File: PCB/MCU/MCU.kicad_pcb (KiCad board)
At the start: 2 copper layers, 40 x 46.2 mm, 36 parts, among them IC1 TMP112NAIDRLR, J1 Conn_02x06_Odd_Even, J2 Conn_02x06_Odd_Even, J3 USB_B_Micro, J4 Programmer, SW1 SW_Push, U1 MPU6050, U2 MDBT50Q-1MV2, U3 MAX6372, Y1 32.768kHz

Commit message: udated by FZ from Windows
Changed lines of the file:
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@@
     (grid_origin 150.16 123.198621)
     (pcbplotparams
-      (layerselection 0x0000020_7ffffffe)
+      (layerselection 0x00010fc_ffffffff)
       (plot_on_all_layers_selection 0x0000000_00000000)
       (disableapertmacros false)
@@
       (sketchpadsonfab false)
       (subtractmaskfromsilk false)
-      (outputformat 3)
+      (outputformat 1)
       (mirror false)
       (drillshape 0)
       (scaleselection 1)
-      (outputdirectory "./")
+      (outputdirectory "Gerber/")
     )
   )
@@
     (fp_line (start 1 0.625) (end -1 0.625)
       (stroke (width 0.1) (type solid)) (layer "F.Fab"))
-    (pad "1" smd roundrect (at -1.0375 0 270) (size 1.175 1.45) (layers "F.Cu" "F.Paste" "F.Mask") (roundrect_rratio 0.212766)
+    (pad "1" smd roundrect (at -1.0375 0 270) (size 1.175 1.45) (layers "F.Cu" "F.Paste" "F.Mask") (roundrect_rratio 0.2127659574)
       (net 7 "+5V") (pintype "passive"))
-    (pad "2" smd roundrect (at 1.0375 0 270) (size 1.175 1.45) (layers "F.Cu" "F.Paste" "F.Mask") (roundrect_rratio 0.212766)
+    (pad "2" smd roundrect (at 1.0375 0 270) (size 1.175 1.45) (layers "F.Cu" "F.Paste" "F.Mask") (roundrect_rratio 0.2127659574)
       (net 1 "GND") (pintype "passive"))
     (model "${KICAD6_3DMODEL_DIR}/Capacitor_SMD.3dshapes/C_0805_2012Metric.wrl"
@@
     (fp_line (start 1 0.625) (end -1 0.625)
       (stroke (width 0.1) (type solid)) (layer "F.Fab"))
-    (pad "1" smd roundrect (at -1.0375 0 270) (size 1.175 1.45) (layers "F.Cu" "F.Paste" "F.Mask") (roundrect_rratio 0.212766)
+    (pad "1" smd roundrect (at -1.0375 0 270) (size 1.175 1.45) (layers "F.Cu" "F.Paste" "F.Mask") (roundrect_rratio 0.2127659574)
       (net 4 "Net-(U2-P0.01{slash}XL2)") (pinfunction "1") (pintype "passive"))
-    (pad "2" smd roundrect (at 1.0375 0 270) (size 1.175 1.45) (layers "F.Cu" "F.Paste" "F.Mask") (roundrect_rratio 0.212766)
+    (pad "2" smd roundrect (at 1.0375 0 270) (size 1.175 1.45) (layers "F.Cu" "F.Paste" "F.Mask") (roundrect_rratio 0.2127659574)
       (net 3 "Net-(U2-P0.00{slash}XL1)") (pinfunction "2") (pintype "passive"))
     (model "${KICAD6_3DMODEL_DIR}/Capacitor_SMD.3dshapes/C_0805_2012Metric.wrl"

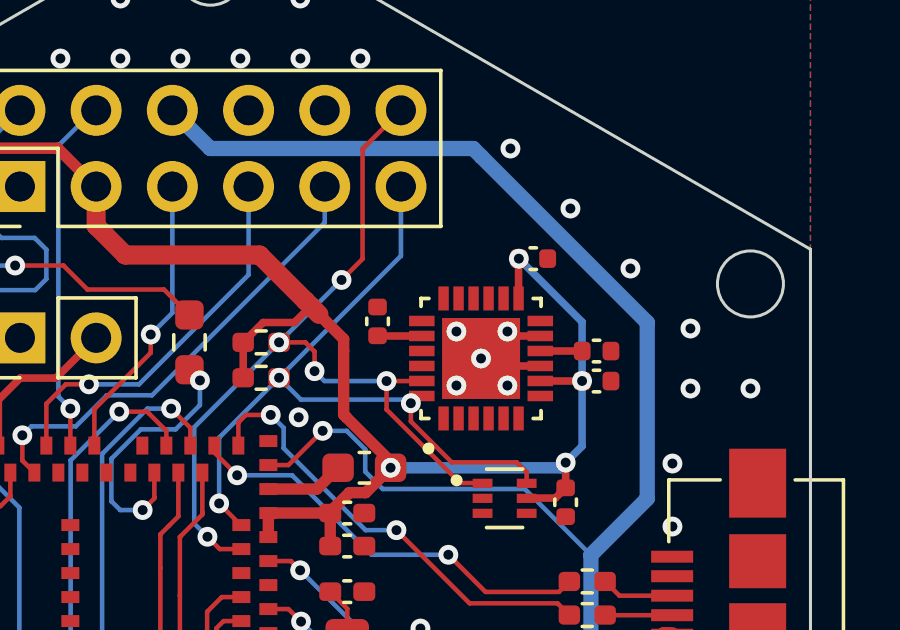
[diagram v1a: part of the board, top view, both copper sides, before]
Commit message: udated by FZ from Windows
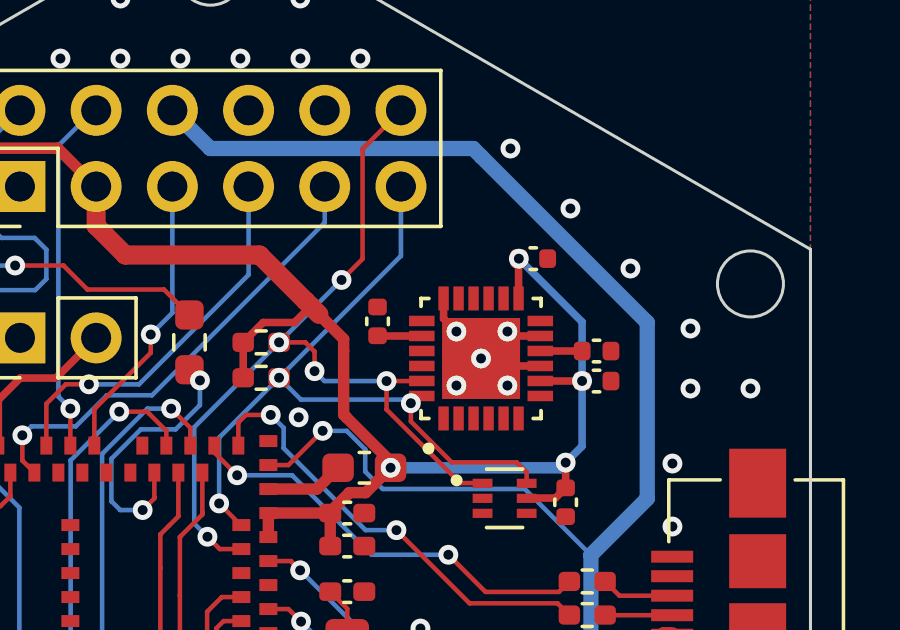
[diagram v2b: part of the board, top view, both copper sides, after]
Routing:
- net GND: track 3.24 -> 4.51 mm
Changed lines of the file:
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@@
   (segment (start 161.155 92.4475) (end 159.43 92.4475) (width 0.254) (layer "F.Cu") (net 1))
   (segment (start 160.208879 91.4475) (end 160.06 91.298621) (width 0.254) (layer "F.Cu") (net 1))
+  (segment (start 157.93 90.1975) (end 157.93 90.868621) (width 0.254) (layer "F.Cu") (net 1))
   (segment (start 159.43 92.4475) (end 159.18 92.1975) (width 0.254) (layer "F.Cu") (net 1))
+  (segment (start 157.93 90.868621) (end 158.36 91.298621) (width 0.254) (layer "F.Cu") (net 1))
   (segment (start 161.155 91.4475) (end 160.208879 91.4475) (width 0.254) (layer "F.Cu") (net 1))
   (via (at 135.16 107.198621) (size 0.6604) (drill 0.3302) (layers "F.Cu" "B.Cu") (free) (net 1))
